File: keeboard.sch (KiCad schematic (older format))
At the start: 24 parts, among them SW1 SW_Push, U1 ATmega32U4-AU, Y1 16MHz

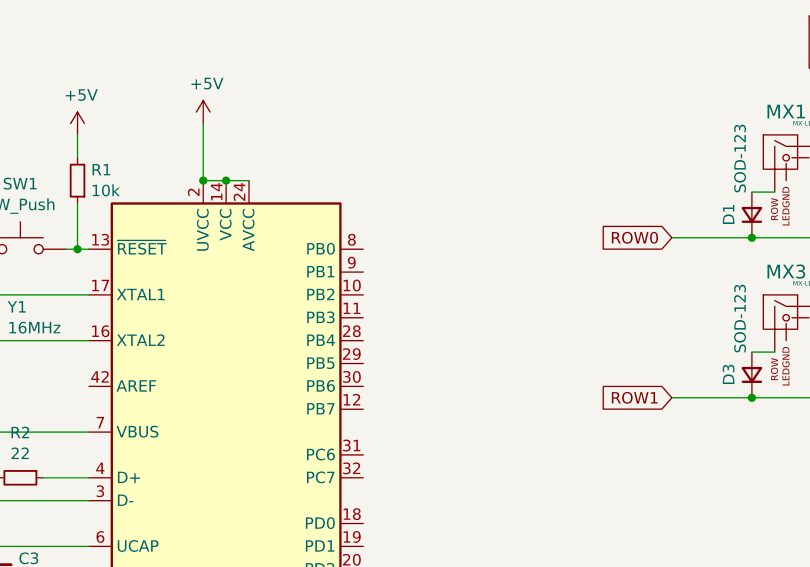
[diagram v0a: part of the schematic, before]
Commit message: finished routing
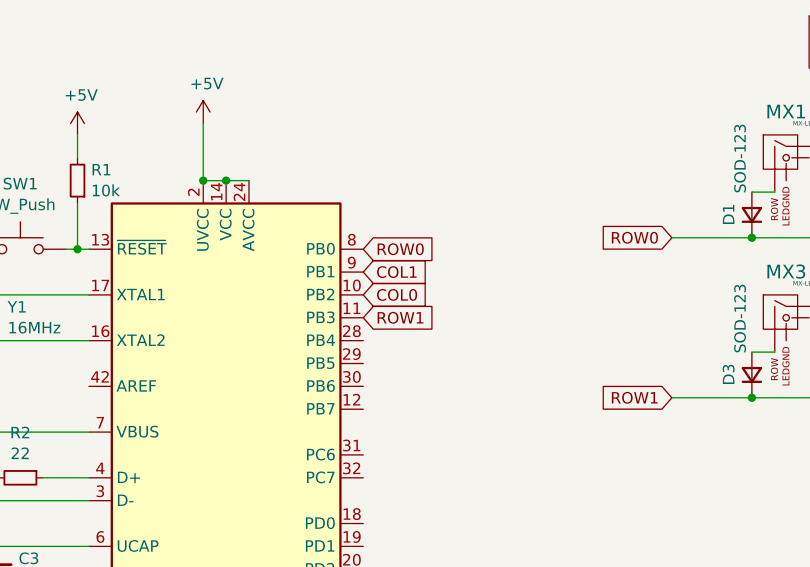
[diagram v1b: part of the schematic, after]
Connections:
- net COL0: now also U1.10 (PB2)
- net COL1: now also U1.9 (PB1)
- net ROW0: now also U1.8 (PB0)
- net ROW1: now also U1.11 (PB3)
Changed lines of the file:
@@
 Wire Wire Line
 	4700 2150 5050 2150
+Text GLabel 3350 1500 2    50   Input ~ 0
+ROW0
+Text GLabel 3350 1800 2    50   Input ~ 0
+ROW1
+Text GLabel 3350 1700 2    50   Input ~ 0
+COL0
+Text GLabel 3350 1600 2    50   Input ~ 0
+COL1
 $EndSCHEMATC
